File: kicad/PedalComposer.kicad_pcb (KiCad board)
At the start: 2 copper layers, 197.6 x 70.1 mm, 82 parts, among them J1 In, J10 AVR-ISP-6, J14 Out, J15 Jack-DC, J2 Send1, J3 Return1, J4 Send2, J5 Return2, J6 Send3, J7 Return3, J8 Send4, J9 Return4, M1 7-SEGMENT-1DIGIT-1INCH-BLUE, SW1 Fx1, SW11 Edit, SW2 Fx2, SW3 Fx3, SW4 Fx4, U1 LM317L_TO92, U10 CD4053B, U2 LM317L_TO92, U20 CD4053B, U3 4543, U30 CD4053B, U5 ATmega8535-16P, Y1 12MHz

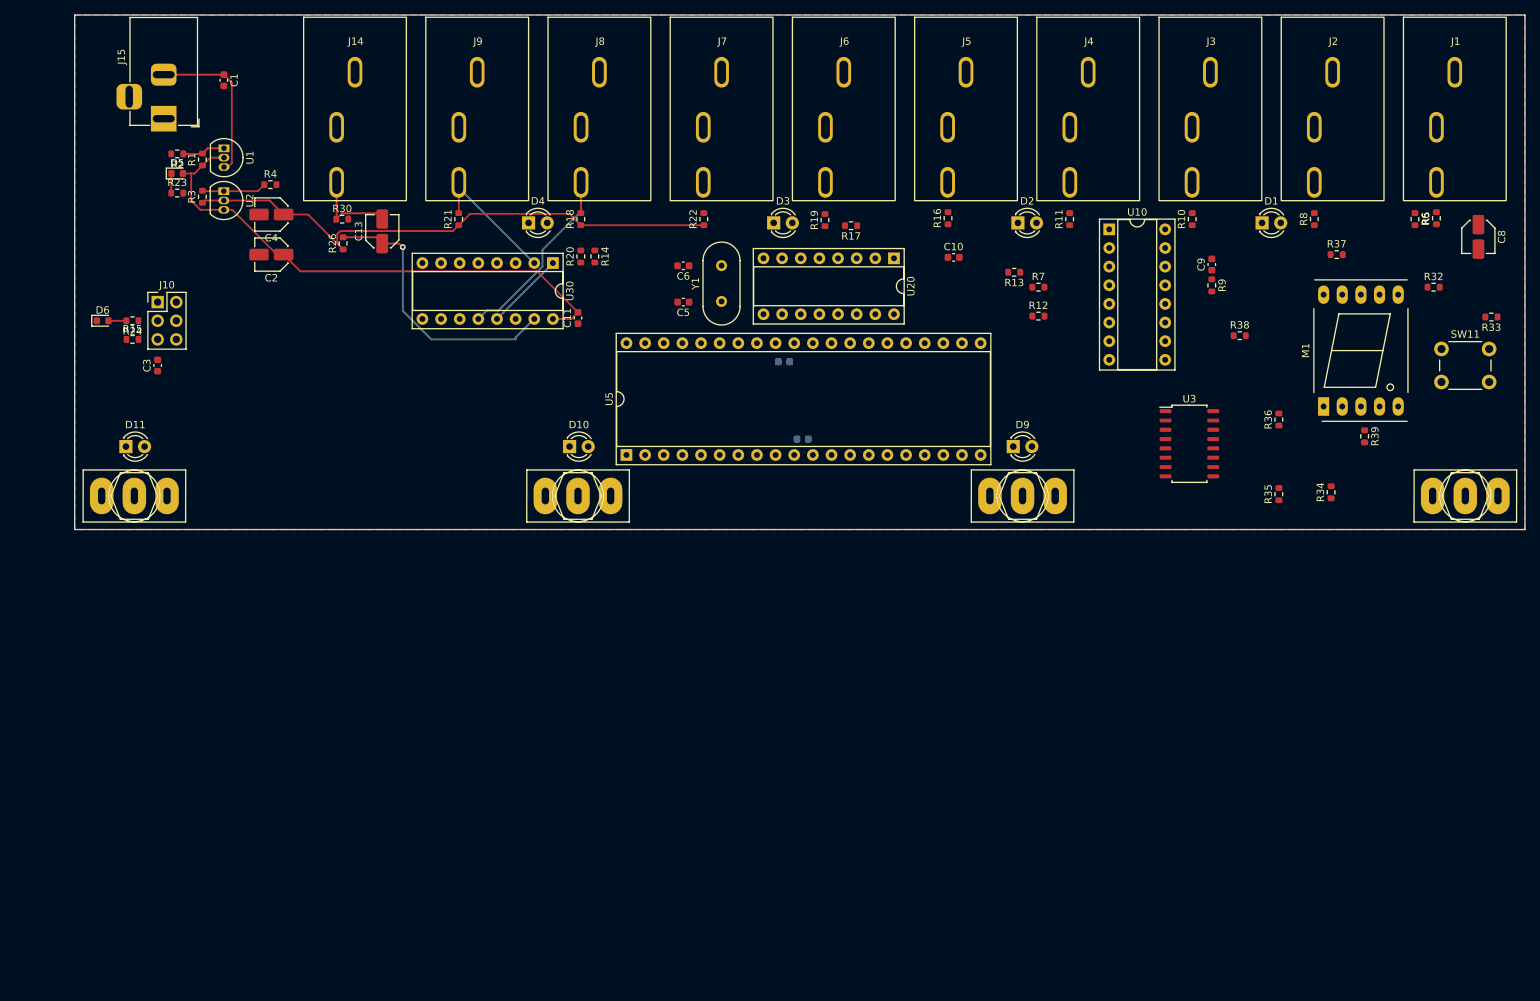
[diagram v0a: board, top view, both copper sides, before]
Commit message: Update PCB
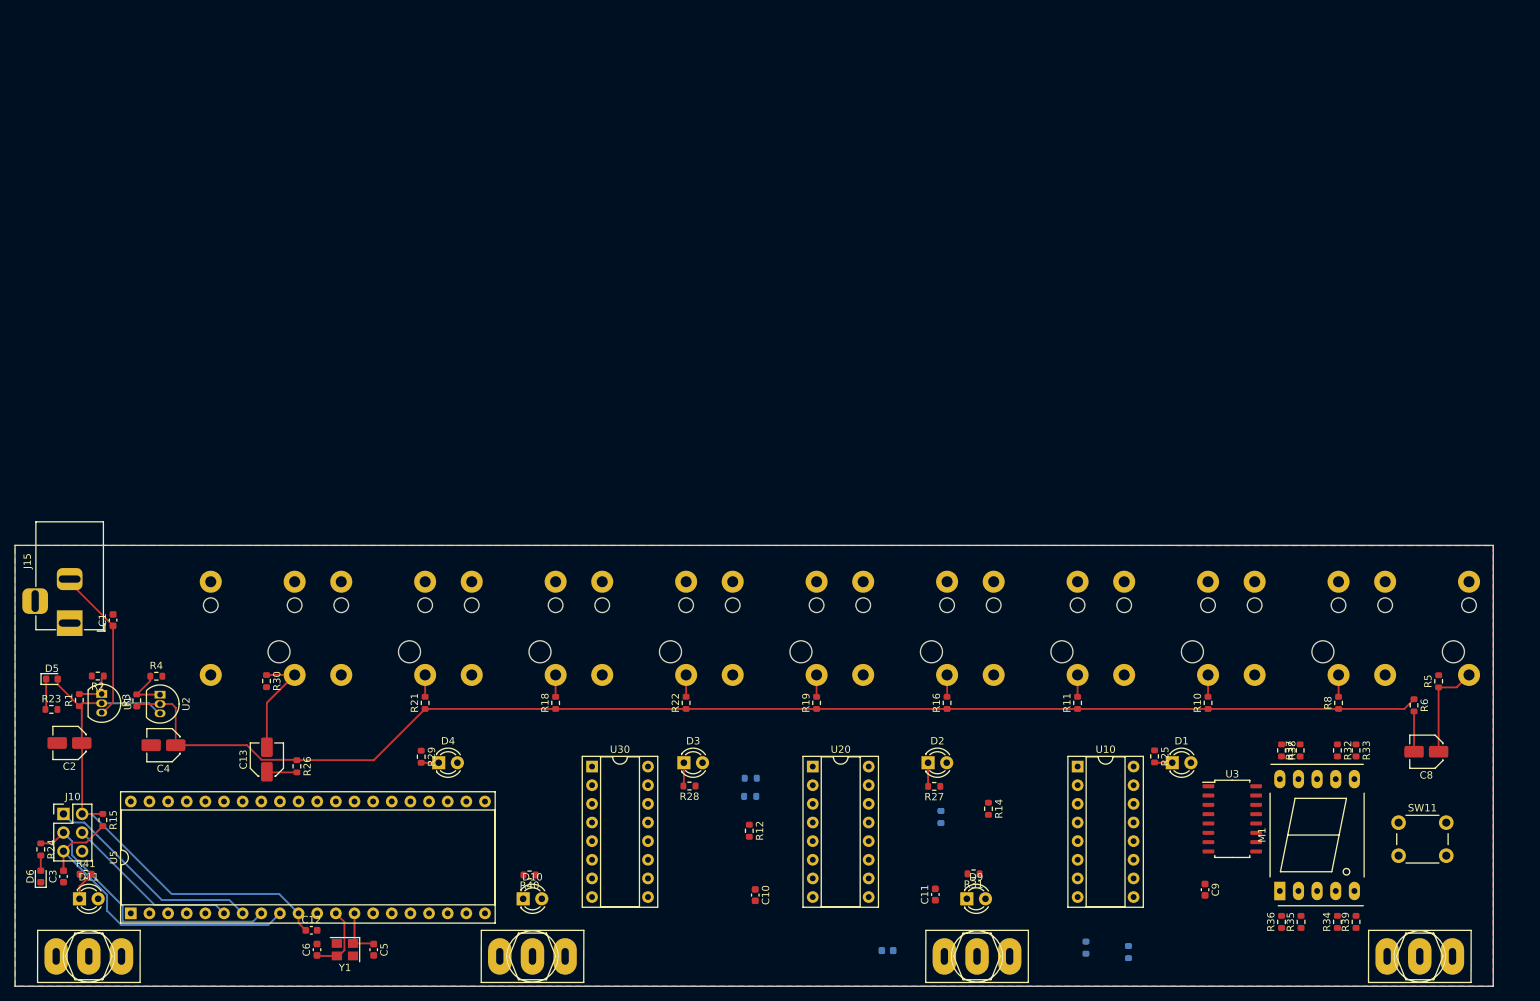
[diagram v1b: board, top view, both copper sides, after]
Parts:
- added R25: 470, Resistor_SMD:R_0603_1608Metric, F.Cu at (188.3, 115.7)
- added R27: 470, Resistor_SMD:R_0603_1608Metric, F.Cu at (158.3, 119.8)
- added R28: 470, Resistor_SMD:R_0603_1608Metric, F.Cu at (124.9, 119.8)
- added R29: 470, Resistor_SMD:R_0603_1608Metric, F.Cu at (88.4, 115.8)
- added R31: 470, Resistor_SMD:R_0603_1608Metric, F.Cu at (163.6, 131.7)
- added R40: 470, Resistor_SMD:R_0603_1608Metric, F.Cu at (103.1, 131.9)
- added R41: 470, Resistor_SMD:R_0603_1608Metric, F.Cu at (42.6, 131.8)
- C12: moved to F.Cu
- C5, C6: value 22pF -> 12pF
- J1, J14, J2, J3, J4, J5, J6, J7, J8, J9: footprint BDMLibrary:Mono Female Socket Connector TS -> BDMLibrary:Jack_6.35mm_Neutrik_NRJ4HF_Horizontal; moved to B.Cu
- R13, R17, R20, R7, R9: moved to B.Cu
- R23: value 10k -> 470
- R24: value 330 -> 470
- Y1: value 12MHz -> 16MHz; footprint Crystal:Crystal_HC49-U_Vertical -> Crystal:Crystal_SMD_3225-4Pin_3.2x2.5mm
- moved C6 105.7 mm to (74.2, 142.1), turned to 90 degrees
- moved Y1 102.2 mm to (78.0, 142.1), turned to 180 degrees
- moved C5 97.8 mm to (81.9, 142.1), turned to -90 degrees
- moved C12 94.7 mm to (73.4, 139.4)
- moved C11 92.4 mm to (158.4, 134.6)
- moved R14 92.4 mm to (165.7, 122.9)
- moved U5 92.0 mm to (48.8, 137.1)
- moved R9 91.9 mm to (178.9, 141.8), turned to 90 degrees
- moved R7 91.4 mm to (184.7, 142.4), turned to 90 degrees
- moved C10 91.0 mm to (133.9, 134.6), turned to -90 degrees
- moved R20 90.8 mm to (159.2, 124.0)
- moved J1 90.1 mm to (231.1, 104.6), turned to 90 degrees
- moved J2 90.0 mm to (213.4, 104.6), turned to 90 degrees
- moved J3 89.9 mm to (195.6, 104.6), turned to 90 degrees
- moved J4 89.8 mm to (177.8, 104.6), turned to 90 degrees
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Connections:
- D1 pad 1: GND -> Net-(D1-Pad1)
- D10 pad 1: GND -> Net-(D10-Pad1)
- D11 pad 1: GND -> Net-(D11-Pad1)
- D2 pad 1: GND -> Net-(D2-Pad1)
- D3 pad 1: GND -> Net-(D3-Pad1)
- D4 pad 1: GND -> Net-(D4-Pad1)
- D9 pad 1: GND -> Net-(D9-Pad1)
- Y1 pad 2: Net-(C6-Pad1) -> GND
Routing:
- net /Vr: track 76.2 -> 183.8 mm
- net /RST: track 0.00 -> 45.0 mm
- net /SCK: track 0.00 -> 38.5 mm
- net Net-(C13-Pad1): track 38.2 -> 4.12 mm, vias 1 -> 0
- net /MISO: track 0.00 -> 30.0 mm
- net Net-(J8-PadT): track 29.6 -> 2.98 mm
- net /MOSI: track 0.00 -> 23.9 mm
- net Net-(J9-PadT): track 19.5 -> 2.96 mm
- net Net-(C8-Pad1): track 0.00 -> 13.6 mm
- net Net-(R20-Pad1): track 10.8 -> 0.00 mm
- net Net-(C6-Pad1): track 0.00 -> 9.60 mm
- net Net-(C5-Pad1): track 0.00 -> 7.03 mm
- net Net-(C8-Pad2): track 0.00 -> 5.50 mm
- net Net-(D11-Pad1): track 0.00 -> 4.04 mm
- net Net-(C13-Pad2): track 12.0 -> 15.3 mm
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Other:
- board size 197.6 x 70.1 mm -> 201.4 x 60.1 mm
